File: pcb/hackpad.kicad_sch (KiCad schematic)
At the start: 4 parts, among them SW1 SW_Push, SW2 SW_Push, SW3 SW_Push, U1 MOUDLE-SEEEDUINO-XIAO

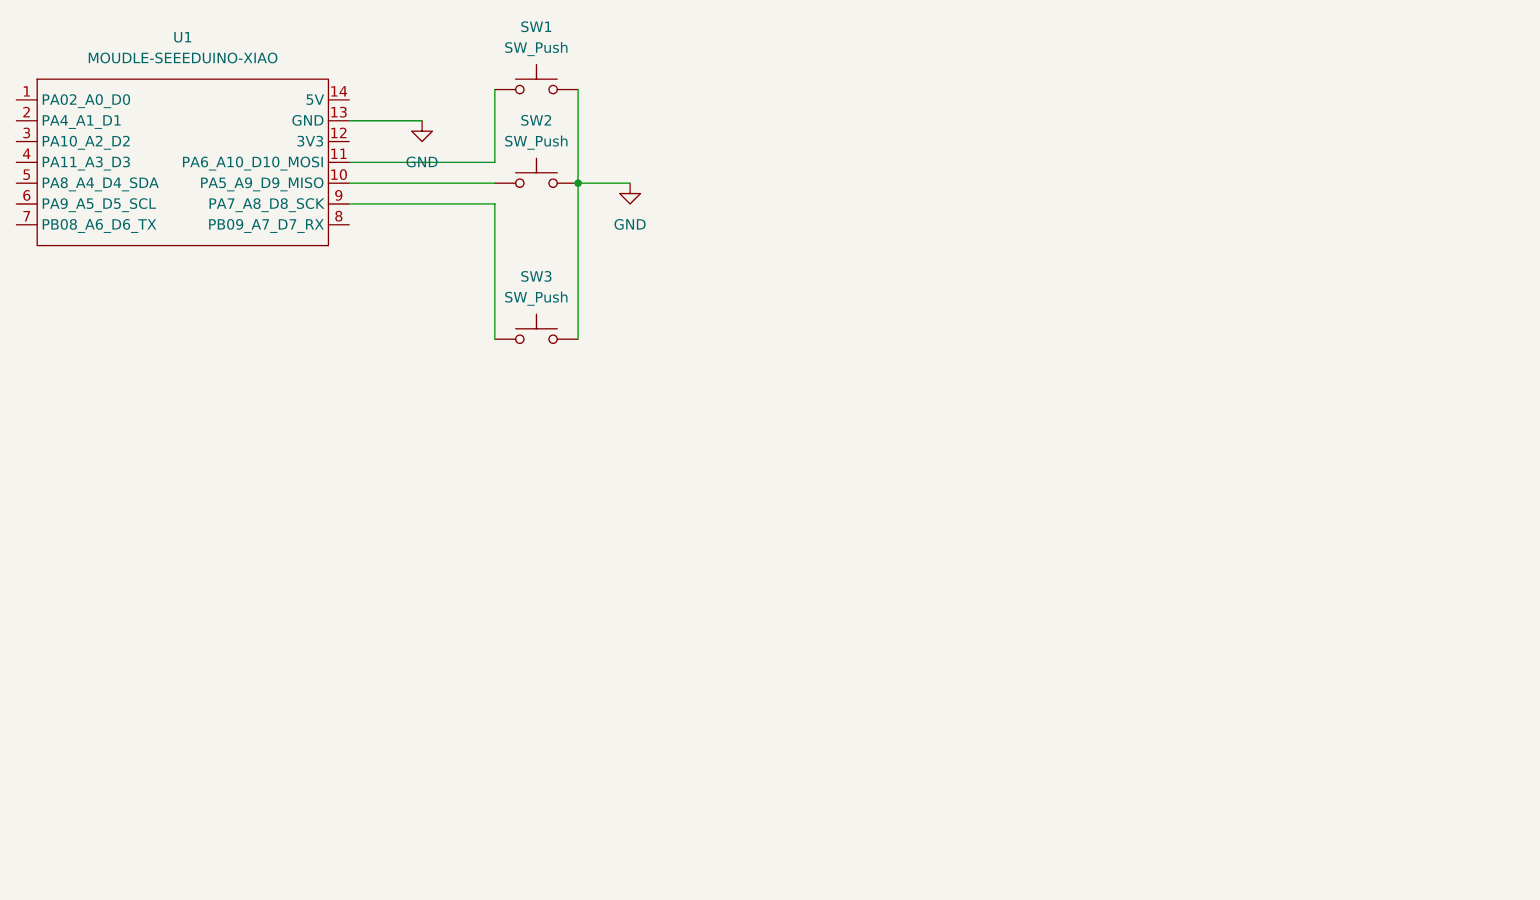
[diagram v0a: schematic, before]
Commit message: Update the schematic
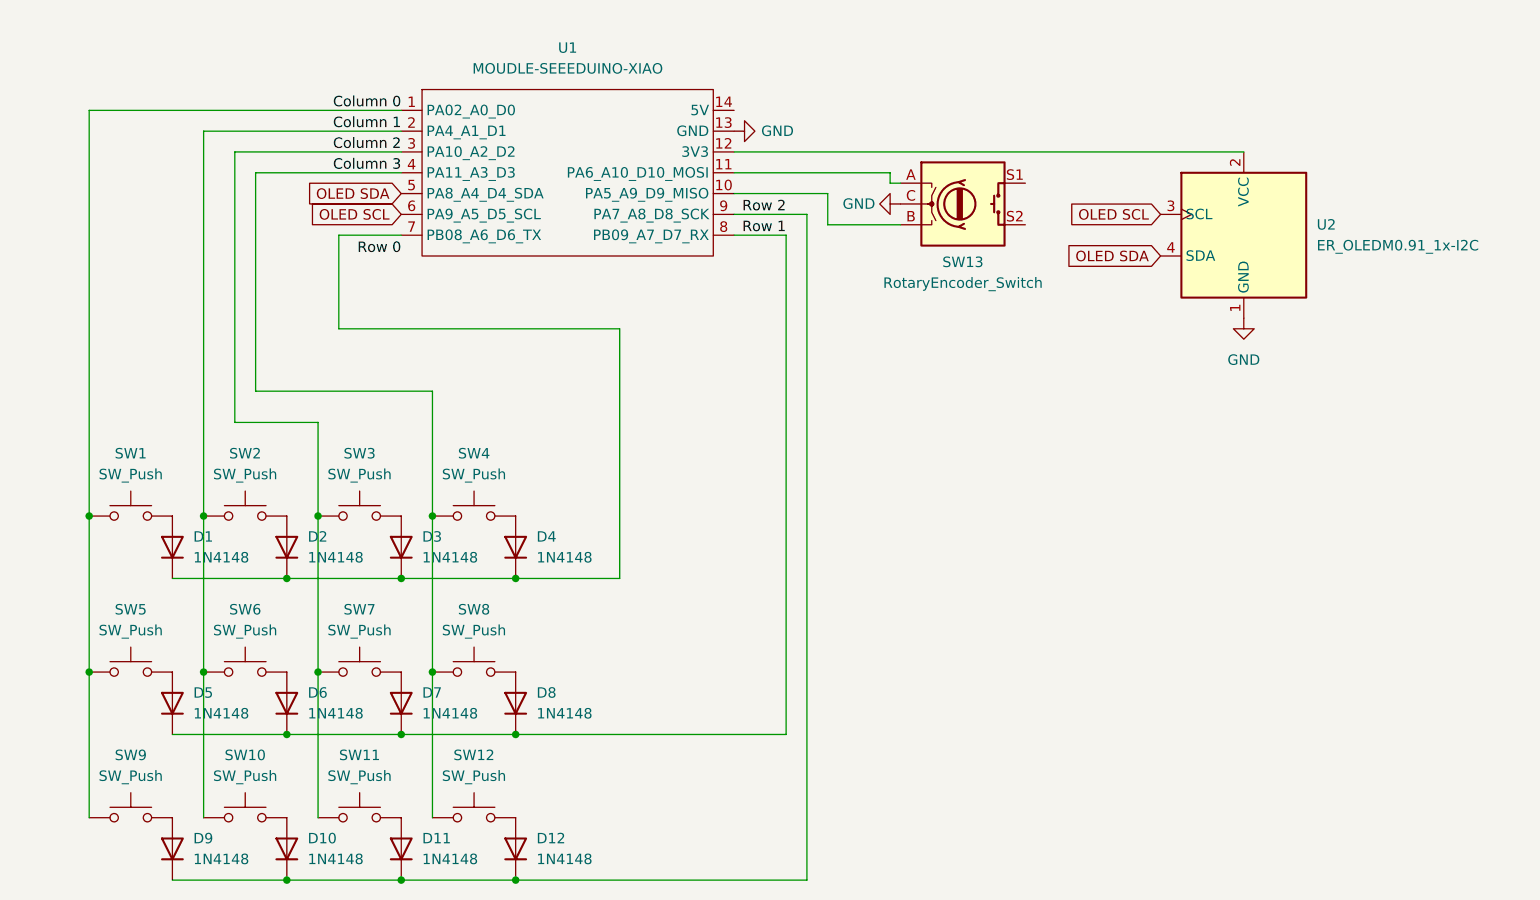
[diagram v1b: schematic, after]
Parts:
- added D1, D10, D11, D12, D2, D3, D4, D5, D6, D7, D8, D9: 1N4148, Diode_THT:D_DO-35_SOD27_P7.62mm_Horizontal, symbol Diode:1N4148
- added SW10, SW11, SW12, SW4, SW5, SW6, SW7, SW8, SW9: SW_Push, Button_Switch_Keyboard:SW_Cherry_MX_1.00u_PCB, symbol Switch:SW_Push
- added SW13: RotaryEncoder_Switch, Rotary_Encoder:RotaryEncoder_Alps_EC11E-Switch_Vertical_H20mm, symbol Device:RotaryEncoder_Switch
- added U2: ER_OLEDM0.91_1x-I2C, Display:ER_OLEDM0.91_1x-I2C, symbol Display_Graphic:ER_OLEDM0.91_1x-I2C
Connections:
- net GND: now also SW13.C, U2.1 (GND); no longer SW1.2, SW2.2, SW3.2
- net at U1.11 (PA6_A10_D10_MOSI): now also SW13.A; no longer SW1.1
- net at U1.10 (PA5_A9_D9_MISO): now also SW13.B; no longer SW2.1
- net Column 0: now reaches U1.1 (PA02_A0_D0)
- net Column 0: now also SW1.1, SW5.1, SW9.1
- net at U1.12 (3V3): now also U2.2 (VCC)
- net Column 1: now reaches U1.2 (PA4_A1_D1)
- net Column 1: now also SW2.1, SW10.1, SW6.1
- net Column 2: now reaches U1.3 (PA10_A2_D2)
- net Column 2: now also SW3.1, SW11.1, SW7.1
- net Column 3: now reaches U1.4 (PA11_A3_D3)
- net Column 3: now also SW12.1, SW4.1, SW8.1
- net OLED SDA: now reaches U1.5 (PA8_A4_D4_SDA)
- net OLED SDA: now also U2.4 (SDA)
- net OLED SCL: now reaches U1.6 (PA9_A5_D5_SCL)
- net OLED SCL: now also U2.3 (SCL)
- net at U1.7 (PB08_A6_D6_TX): now also D1.1 (K), D2.1 (K), D3.1 (K), D4.1 (K)
- net Row 1: now reaches U1.8 (PB09_A7_D7_RX)
- net Row 1: now also D5.1 (K), D6.1 (K), D7.1 (K), D8.1 (K)
- net Row 2: now reaches U1.9 (PA7_A8_D8_SCK)
- net Row 2: now also D10.1 (K), D11.1 (K), D12.1 (K), D9.1 (K); no longer SW3.1
- new net: D12.2 (A), SW12.2
- new net: D8.2 (A), SW8.2
- new net: D11.2 (A), SW11.2
- new net: D1.2 (A), SW1.2
- new net: D9.2 (A), SW9.2
- new net: D4.2 (A), SW4.2
- new net: D10.2 (A), SW10.2
- new net: D5.2 (A), SW5.2
- new net: D2.2 (A), SW2.2
- new net: D3.2 (A), SW3.2
- new net: D7.2 (A), SW7.2
- new net: D6.2 (A), SW6.2
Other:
- moved on the sheet: SW1, SW2, SW3, U1
